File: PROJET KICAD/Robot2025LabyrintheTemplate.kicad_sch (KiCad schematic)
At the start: 35 parts, among them J1 HC-SR04 gauche, J11 SERVO MOTEUR 4, J13 capteur TOF BAS, J14 Vinput regul, J15 CON 1x2 POLARIZED, J16 capteur TOF HAUT, J17 moteur 2 AV, J18 Vout regul, J2 cap sen0101, J20 moteur 3 DR, J21 moteur 4 DR, J22 moteur 1 AV, J3 SERVO MOTEUR 1, J4 SERVO MOTEUR 2, J6 cap sen0101, J7 SERVO MOTEUR 3, J8 HC-SR04 droite, U1 module_mpu6050, U2 LM1117MPX-3.3, U4 NRF24L01P-Module-E01ML01DP5_B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

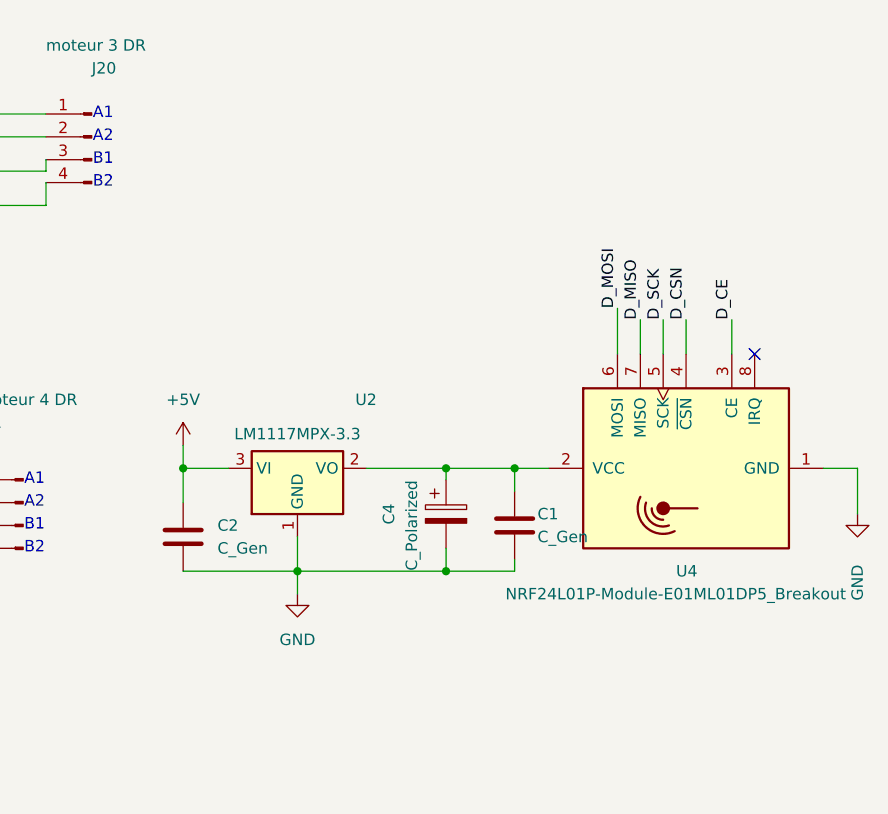
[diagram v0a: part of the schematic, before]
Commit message: maj2
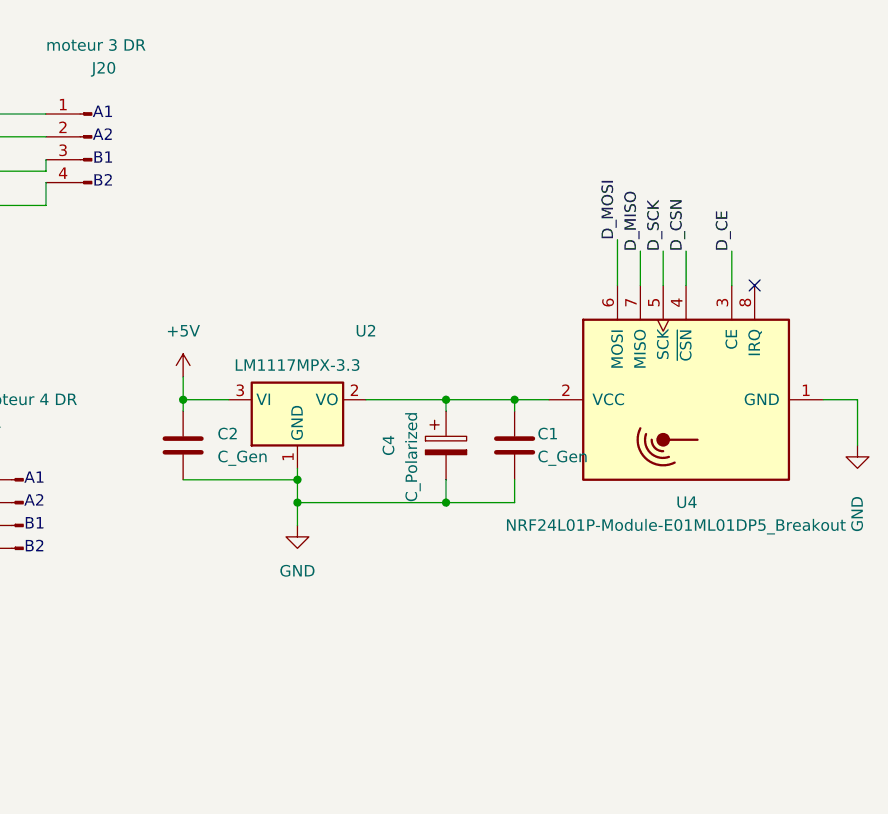
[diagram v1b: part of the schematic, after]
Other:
- moved on the sheet: C1, C2, C4, U2, U4
